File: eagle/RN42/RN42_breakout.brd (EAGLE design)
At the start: 38.8 x 20.8 mm, 15 parts

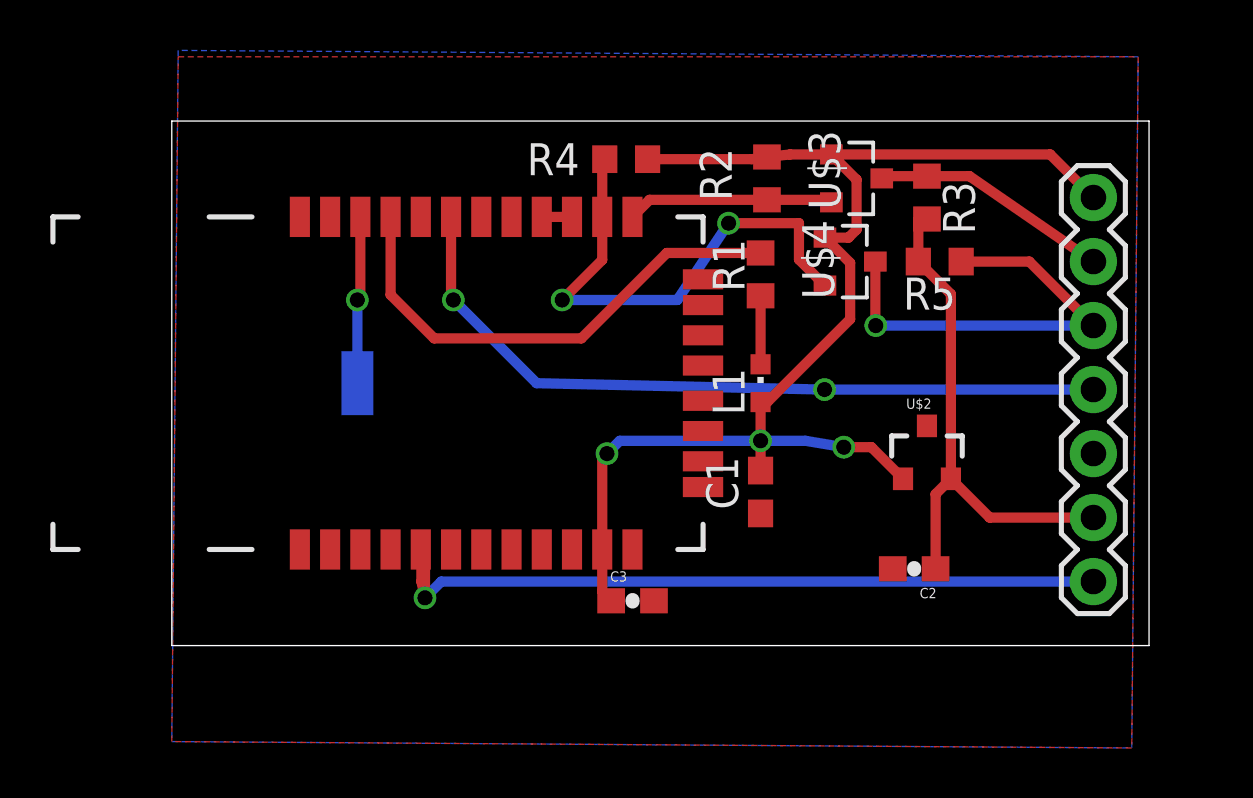
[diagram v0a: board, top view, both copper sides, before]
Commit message: Update RN42 breakout board.
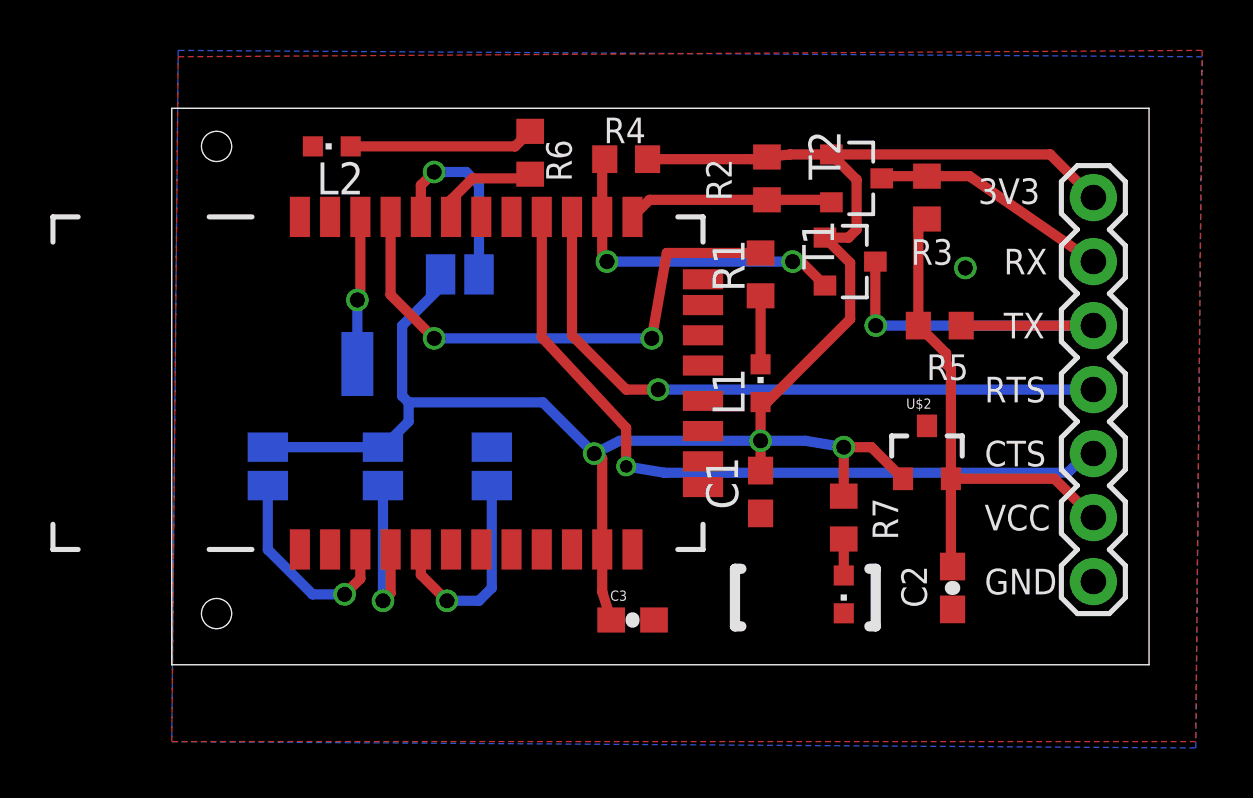
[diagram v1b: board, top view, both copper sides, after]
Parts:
- added L2, L3: (no value), led:CHIPLED_0603
- added R6, R7: 1k, rcl:R0603
- added SJ1, SJ2, SJ3, SJ4: (no value), jumper:SJ
- T1: value N-CHANNEL-MOSFET-BSS138 -> N-MOSFET
- moved R5 2.54 mm to (35.3, 16.3)
- moved C2 1.70 mm to (35.8, 5.84), turned to 270 degrees
- moved C3 0.76 mm to (23.1, 4.57)
- moved FACTORY_RST 0.76 mm to (12.2, 14.7)
- renumbered U$3 to T2, U$4 to T1
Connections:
- removed net LINK: U$1.15, U$1.16
- new net AUTODISCOVERY: SJ3.1, U$1.20
- new net BD_RATE: SJ4.1, U$1.4
- new net BT_MASTER: SJ1.1, U$1.3
- new net CTS: J1.3, U$1.16
- new net N$3: L2.A, R6.2
- new net N$4: L3.A, R7.1
- new net RTS: J1.4, U$1.15
- net 3V3: now also R7.2, SJ1.2, SJ3.2, SJ4.2
- net GND: now also J1.1, L2.C, L3.C, SJ2.2; no longer J1.3, U$1.4
- net RESET: now also SJ2.1; no longer J1.1
- net STATUS: now also R6.1; no longer J1.4
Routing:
- net CTS: track 0.00 -> 30.1 mm, vias 0 -> 1
- net RTS: track 0.00 -> 26.3 mm, vias 0 -> 1
- net STATUS: track 30.1 -> 4.24 mm, vias 2 -> 0
- net 3V3: track 53.3 -> 77.3 mm
- net RESET: track 30.7 -> 8.52 mm
- net BT_MASTER: track 0.00 -> 8.37 mm, vias 0 -> 1
- net AUTODISCOVERY: track 0.00 -> 7.55 mm, vias 0 -> 1
- net N$3: track 0.00 -> 7.37 mm
- net TX: track 20.2 -> 13.3 mm
- net BD_RATE: track 0.00 -> 6.73 mm, vias 0 -> 1
- net N$4: track 0.00 -> 1.45 mm
- net N$2: track 19.9 -> 21.3 mm, vias 0 -> 2
- net LINK: track 1.20 -> 0.00 mm
- net TXH: track 17.5 -> 16.4 mm
- net FACTORY_RST: track 6.65 -> 5.89 mm
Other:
- board size 38.8 x 20.8 mm -> 38.8 x 22.1 mm
- board text added: "3V3"
- board text added: "CTS"
- board text added: "PWR"
- board text added: "RTS"
- board text removed: "3.3V"
- board text removed: "STA"
- board text removed: "nRST"
